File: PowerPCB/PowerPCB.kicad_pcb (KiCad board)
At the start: 2 copper layers, 71.8 x 92.4 mm, 41 parts, among them J1 Conn_01x03_Male, J2 Conn_01x10_Male, J5 Conn_01x07_Male, K1 1721081-5, K2 1721081-5, K3 1721081-5, Q1 Q_PMOS_DGS, U1 NCP1117-3.3_SOT223, U2 STM32F413ZHTx, U3 NCP1117-5.0_SOT223, U4 MCP2562-E-P, U5 MCP2562-E-P

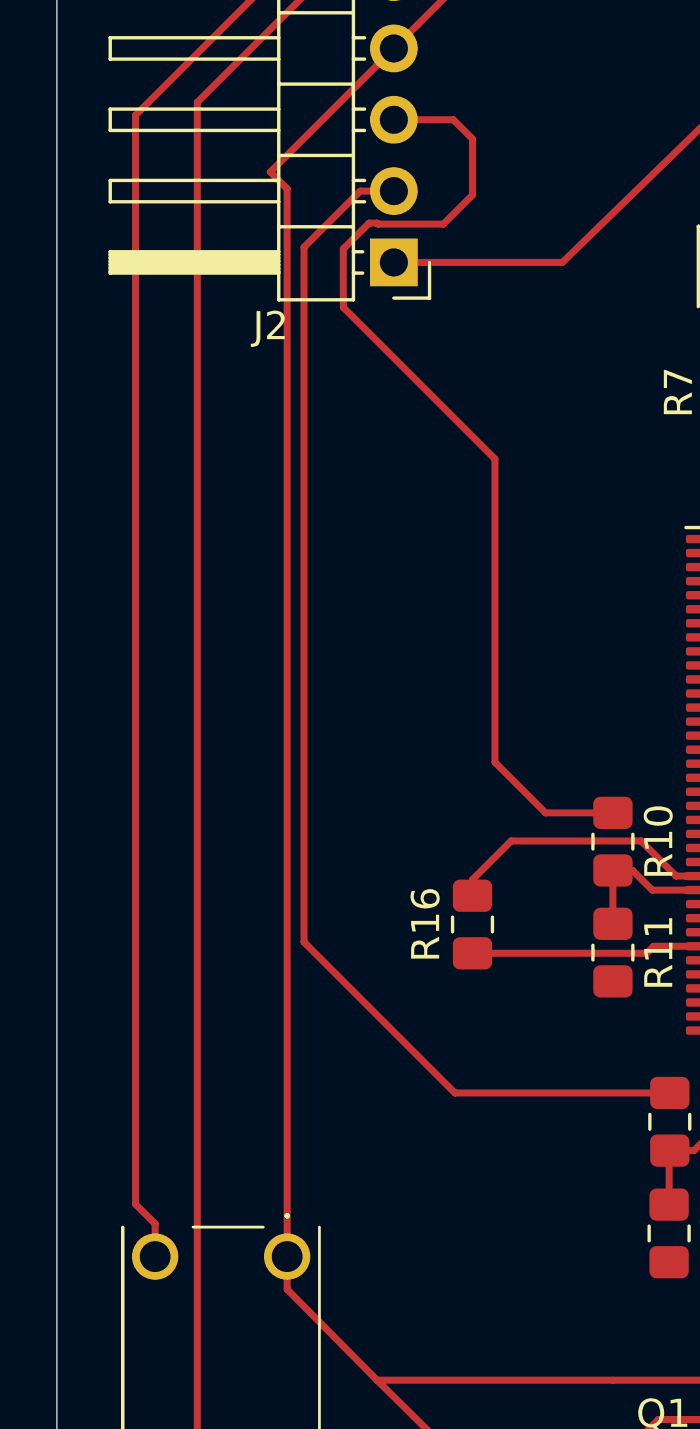
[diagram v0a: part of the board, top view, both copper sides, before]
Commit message: small changes to tracks
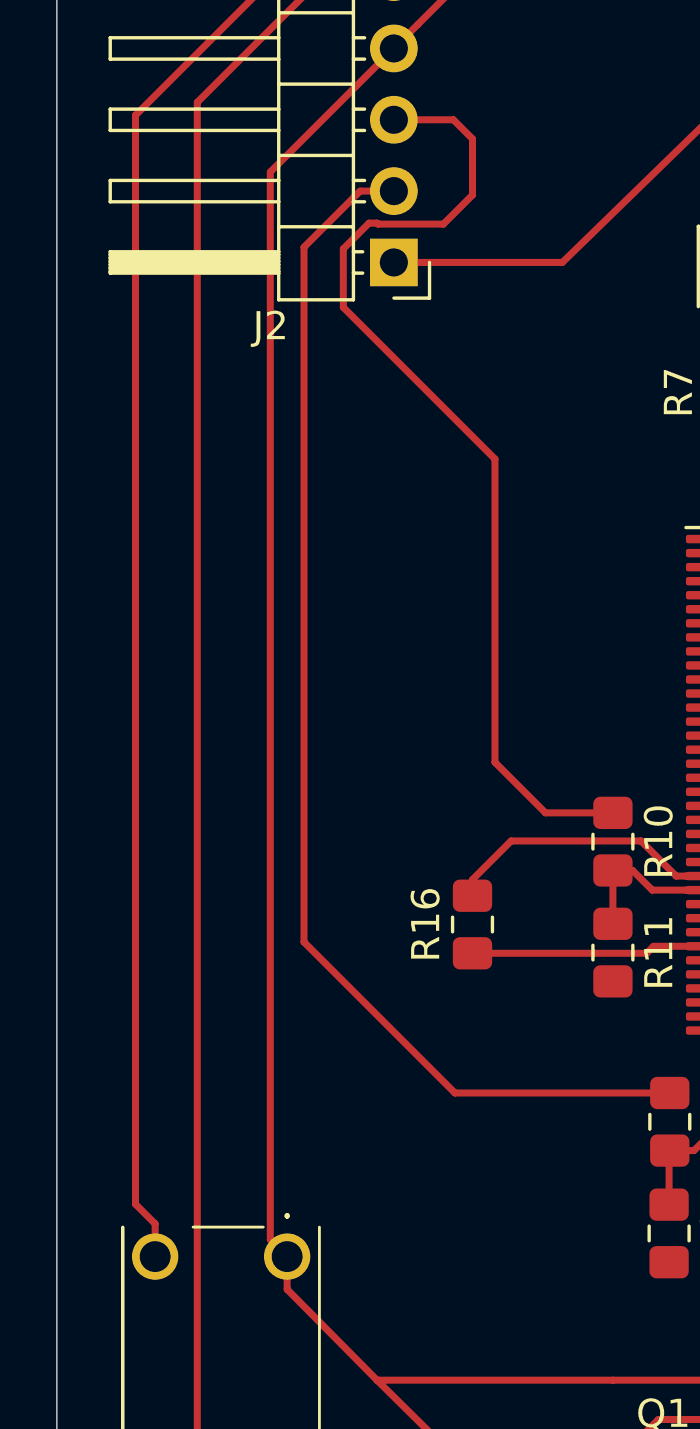
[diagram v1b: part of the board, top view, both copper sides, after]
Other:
- net class Default: trace_width 0.25 -> 1.27
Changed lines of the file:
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@@
   )
   (setup
-    (last_trace_width 0.25)
+    (last_trace_width 1.27)
     (trace_clearance 0.2)
     (zone_clearance 0.508)
@@
   (net_class Default "This is the default net class."
     (clearance 0.2)
-    (trace_width 0.25)
+    (trace_width 1.27)
     (via_dia 0.8)
     (via_drill 0.4)
@@
   (segment (start 374.4 184.2) (end 376.2 182.4) (width 0.25) (layer F.Cu) (net 2))
   (segment (start 376.2 182.4) (end 376.2 176) (width 0.25) (layer F.Cu) (net 2))
-  (segment (start 345.2 187.78) (end 340.8 192.18) (width 0.25) (layer F.Cu) (net 2))
   (segment (start 362.9 239.3) (end 364.675 239.3) (width 0.25) (layer F.Cu) (net 2))
   (segment (start 361.2 241) (end 362.9 239.3) (width 0.25) (layer F.Cu) (net 2))
@@
   (segment (start 356.13 238.4) (end 359.8 238.4) (width 0.25) (layer F.Cu) (net 2))
   (segment (start 359.8 238.4) (end 360.15 238.05) (width 0.25) (layer F.Cu) (net 2))
-  (segment (start 341.4 192.78) (end 341.4 230.8) (width 0.25) (layer F.Cu) (net 2))
-  (segment (start 340.8 192.18) (end 341.4 192.78) (width 0.25) (layer F.Cu) (net 2))
   (segment (start 374.4 184.2) (end 348.78 184.2) (width 0.25) (layer F.Cu) (net 2))
   (segment (start 346.049999 186.930001) (end 345.2 187.78) (width 0.25) (layer F.Cu) (net 2))
   (segment (start 348.78 184.2) (end 346.049999 186.930001) (width 0.25) (layer F.Cu) (net 2))
+  (segment (start 340.8 230.2) (end 341.4 230.8) (width 0.25) (layer F.Cu) (net 2))
+  (segment (start 345.2 187.78) (end 340.8 192.18) (width 0.25) (layer F.Cu) (net 2))
+  (segment (start 340.8 192.18) (end 340.8 230.2) (width 0.25) (layer F.Cu) (net 2))
   (segment (start 362 230) (end 362 232) (width 0.25) (layer F.Cu) (net 3))
   (segment (start 362 197) (end 362 199) (width 0.25) (layer F.Cu) (net 4))
